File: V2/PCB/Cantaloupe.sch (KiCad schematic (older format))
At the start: 121 parts, among them J1 USB_In, J2 OLED, J3 Link, J4 Debug, J5 Trackball, Q1 2N7002, Q2 AO3401A, SW1 MX, SW10 MX, SW11 MX, SW12 MX, SW13 MX, SW14 MX, SW15 MX, SW16 MX, SW17 MX, SW18 MX, SW19 MX, SW2 MX, SW20 MX, SW21 MX, SW22 MX, SW23 MX, SW24 MX, SW25 MX, SW26 MX, SW27 MX, SW28 MX, SW29 MX, SW3 MX, SW30 MX, SW31 Encoder, SW32 MX, SW4 MX, SW5 MX, SW6 MX, SW7 MX, SW8 MX, SW9 MX, U1 STM32F4x1CxUx, U2 SRV0504, U3 SRV0504, U4 XC6206P332MR, U5 LMV321, Y1 8MHz

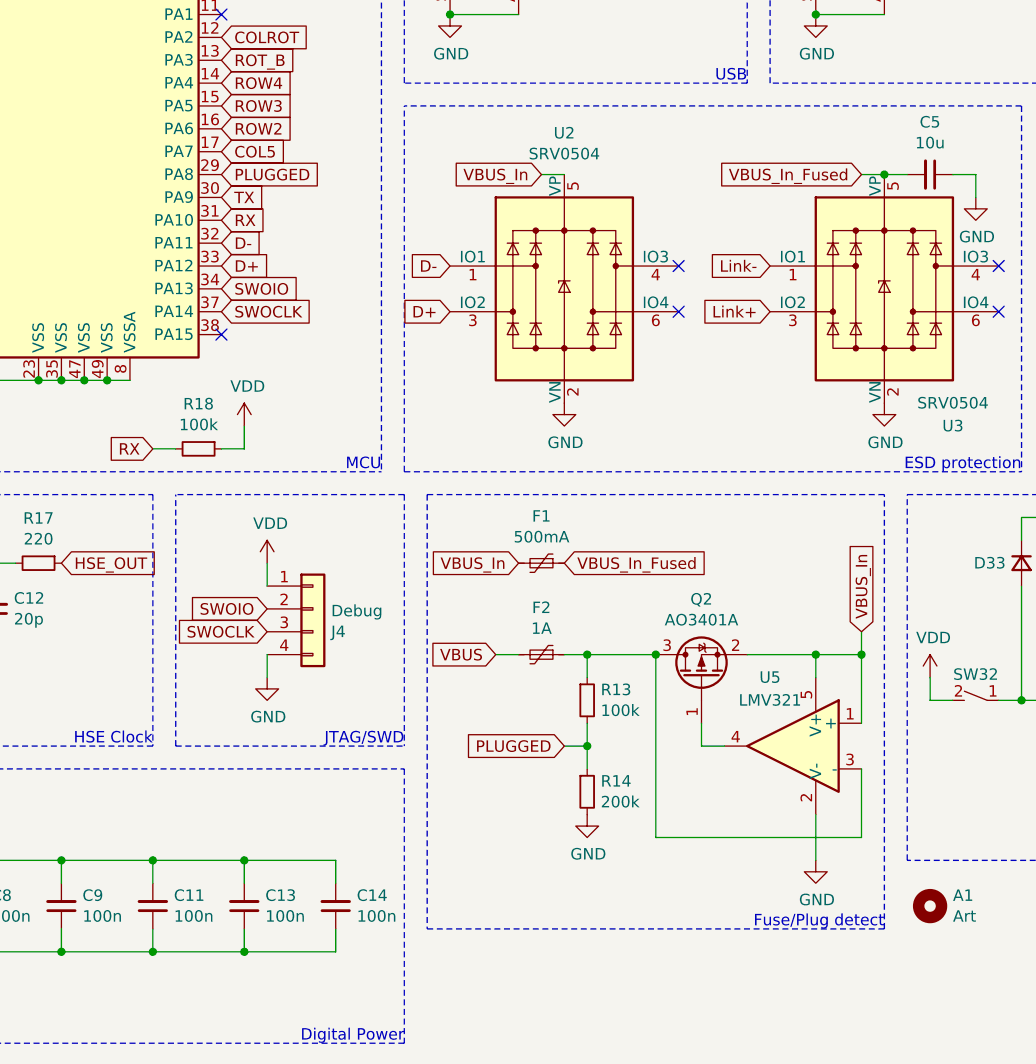
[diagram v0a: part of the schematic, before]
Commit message: Clean up of design. Added gerbers and files for FR4 plates.
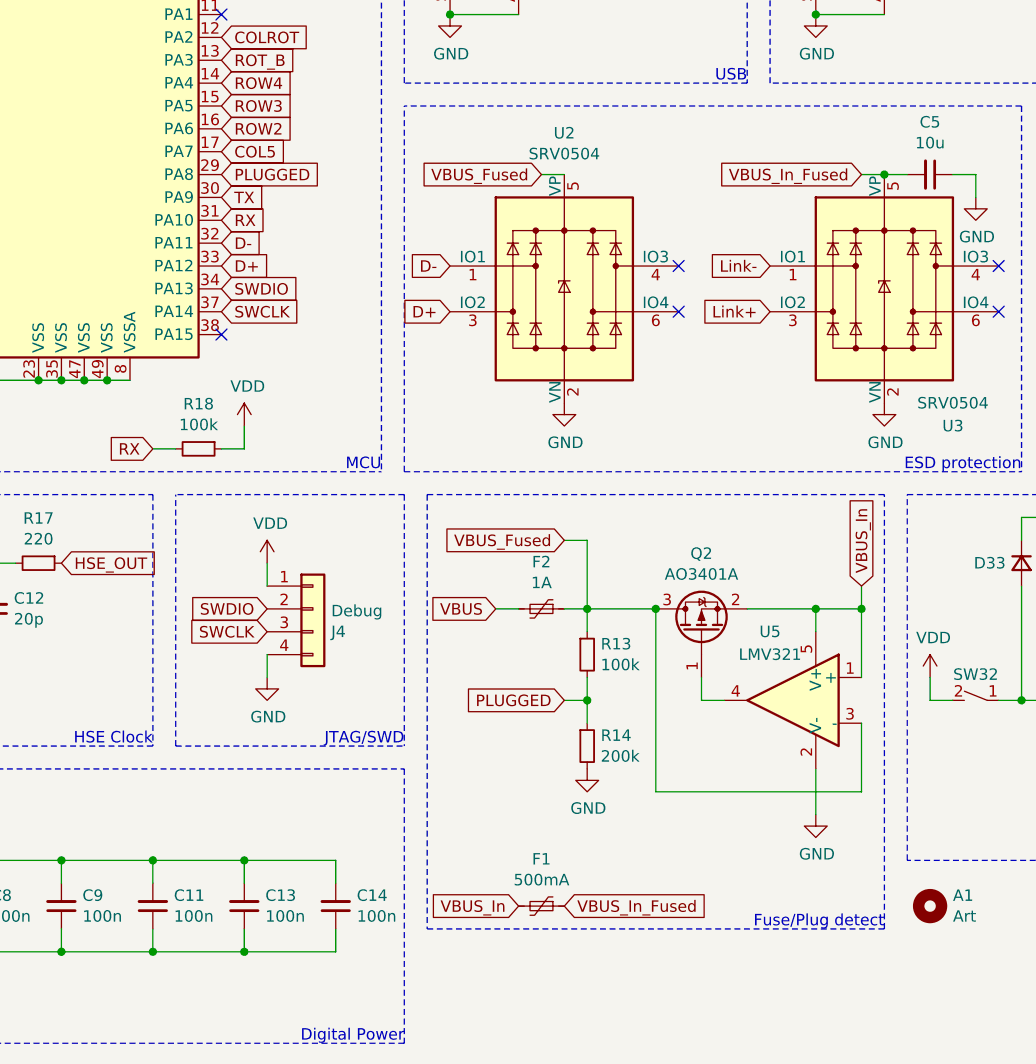
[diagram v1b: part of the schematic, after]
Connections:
- net VBUS_In: no longer U2.5 (VP)
- net VBUS_Fused: now reaches F2.1, Q2.3 (D), R13.1, U5.3 (-)
- net VBUS_Fused: now also U2.5 (VP)
- net SWOCLK renamed SWCLK
- net SWOIO renamed SWDIO
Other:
- moved on the sheet: F1, F2, Q2, R13, R14, U5
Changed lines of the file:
@@
 Wire Notes Line
 	2100 5800 6400 5800
-Text GLabel 6900 4900 0    50   Input ~ 0
+Text GLabel 6900 6400 0    50   Input ~ 0
 VBUS_In
 $Comp
 L Device:Polyfuse_Small F1
 U 1 1 6233E288
-P 7000 4900
-F 0 "F1" V 6795 4900 50  0000 C CNN
-F 1 "500mA" V 6886 4900 50  0000 C CNN
-F 2 "Fuse:Fuse_1206_3216Metric" H 7050 4700 50  0001 L CNN
-F 3 "~" H 7000 4900 50  0001 C CNN
-	1    7000 4900
+P 7000 6400
+F 0 "F1" V 6795 6400 50  0000 C CNN
+F 1 "500mA" V 6886 6400 50  0000 C CNN
+F 2 "Fuse:Fuse_1206_3216Metric" H 7050 6200 50  0001 L CNN
+F 3 "~" H 7000 6400 50  0001 C CNN
+	1    7000 6400
 	0    1    1    0
 $EndComp
-Text GLabel 7100 4900 2    50   Input ~ 0
+Text GLabel 7100 6400 2    50   Input ~ 0
 VBUS_In_Fused
 Text GLabel 9200 800  2    50   Input ~ 0
@@
 	4400 1000 4800 1000
 Text GLabel 5600 3700 2    50   Input ~ 0
-SWOIO
+SWDIO
 $Comp
 L MCU_ST_STM32F4:STM32F411CCUx U1
@@
 	10100 5200 10000 5200
 Text GLabel 5600 3800 2    50   Input ~ 0
-SWOCLK
+SWCLK
 NoConn ~ 5600 3900
 NoConn ~ 4300 2800
-Text GLabel 5800 5100 0    50   Input ~ 0
-SWOIO
-Text GLabel 5800 5200 0    50   Input ~ 0
-SWOCLK
 Wire Notes Line
 	6400 4600 5400 4600
@@
 NoConn ~ 9000 3600
 Text GLabel 7000 3200 0    50   Input ~ 0
-VBUS_In
+VBUS_Fused
 Connection ~ 8500 3200
 Wire Wire Line
@@
 Wire Notes Line
 	8500 6500 8500 4600
-Text GLabel 8400 5200 1    50   Input ~ 0
+Text GLabel 8400 5000 1    50   Input ~ 0
 VBUS_In
 Wire Wire Line
-	7700 5700 7700 5600
+	7700 5500 7700 5400
 $Comp
 L Transistor_FET:AO3401A Q2
 U 1 1 62437866
-P 7700 5400
-F 0 "Q2" V 8042 5400 50  0000 C CNN
-F 1 "AO3401A" V 7951 5400 50  0000 C CNN
-F 2 "Package_TO_SOT_SMD:SOT-23" H 7900 5325 50  0001 L CIN
-F 3 "http://www.aosmd.com/pdfs/datasheet/AO3401A.pdf" H 7700 5400 50  0001 L CNN
-	1    7700 5400
+P 7700 5200
+F 0 "Q2" V 8042 5200 50  0000 C CNN
+F 1 "AO3401A" V 7951 5200 50  0000 C CNN
+F 2 "Package_TO_SOT_SMD:SOT-23" H 7900 5125 50  0001 L CIN
+F 3 "http://www.aosmd.com/pdfs/datasheet/AO3401A.pdf" H 7700 5200 50  0001 L CNN
+	1    7700 5200
 	0    -1   -1   0
 $EndComp
 Wire Wire Line
-	7800 5700 7700 5700
-Wire Wire Line
-	7500 6100 8400 6100
+	7800 5500 7700 5500
+Wire Wire Line
+	7500 5900 8400 5900
 $Comp
 L power:GND #PWR0123
 U 1 1 631C4FB0
-P 8200 6200
-F 0 "#PWR0123" H 8200 5950 50  0001 C CNN
-F 1 "GND" H 8205 6027 50  0000 C CNN
-F 2 "" H 8200 6200 50  0001 C CNN
-F 3 "" H 8200 6200 50  0001 C CNN
-	1    8200 6200
-	1    0    0    -1
-$EndComp
-Wire Wire Line
-	8400 5200 8400 5300
-Connection ~ 8400 5300
-Wire Wire Line
-	8400 5800 8400 6100
-Wire Wire Line
-	8400 5600 8400 5300
-Wire Wire Line
-	7900 5300 8200 5300
-Connection ~ 8200 5300
-Wire Wire Line
-	8200 5300 8400 5300
-Wire Wire Line
-	8200 5400 8200 5300
-Wire Wire Line
-	8200 6000 8200 6200
-Wire Wire Line
-	7500 5300 7500 6100
+P 8200 6000
+F 0 "#PWR0123" H 8200 5750 50  0001 C CNN
+F 1 "GND" H 8205 5827 50  0000 C CNN
+F 2 "" H 8200 6000 50  0001 C CNN
+F 3 "" H 8200 6000 50  0001 C CNN
+	1    8200 6000
+	1    0    0    -1
+$EndComp
+Wire Wire Line
+	8400 5000 8400 5100
+Connection ~ 8400 5100
+Wire Wire Line
+	8400 5600 8400 5900
+Wire Wire Line
+	8400 5400 8400 5100
+Wire Wire Line
+	7900 5100 8200 5100
+Connection ~ 8200 5100
+Wire Wire Line
+	8200 5100 8400 5100
+Wire Wire Line
+	8200 5200 8200 5100
+Wire Wire Line
+	8200 5800 8200 6000
+Wire Wire Line
+	7500 5100 7500 5900
 $Comp
 L Amplifier_Operational:LMV321 U5
 U 1 1 62452FE5
-P 8100 5700
-F 0 "U5" H 8200 6000 50  0000 C CNN
-F 1 "LMV321" H 8200 5900 50  0000 C CNN
-F 2 "Package_TO_SOT_SMD:SOT-23-5" H 8100 5700 50  0001 L CNN
-F 3 "http://www.ti.com/lit/ds/symlink/lmv324.pdf" H 8100 5700 50  0001 C CNN
-	1    8100 5700
+P 8100 5500
+F 0 "U5" H 8200 5800 50  0000 C CNN
+F 1 "LMV321" H 8200 5700 50  0000 C CNN
+F 2 "Package_TO_SOT_SMD:SOT-23-5" H 8100 5500 50  0001 L CNN
+F 3 "http://www.ti.com/lit/ds/symlink/lmv324.pdf" H 8100 5500 50  0001 C CNN
+	1    8100 5500
 	-1   0    0    -1
 $EndComp
@@
 L Device:Polyfuse_Small F2
 U 1 1 6240F7C8
-P 7000 5300
-F 0 "F2" V 6795 5300 50  0000 C CNN
-F 1 "1A" V 6886 5300 50  0000 C CNN
-F 2 "Fuse:Fuse_1206_3216Metric" H 7050 5100 50  0001 L CNN
-F 3 "~" H 7000 5300 50  0001 C CNN
-	1    7000 5300
+P 7000 5100
+F 0 "F2" V 6795 5100 50  0000 C CNN
+F 1 "1A" V 6886 5100 50  0000 C CNN
+F 2 "Fuse:Fuse_1206_3216Metric" H 7050 4900 50  0001 L CNN
+F 3 "~" H 7000 5100 50  0001 C CNN
+	1    7000 5100
 	0    1    1    0
 $EndComp
 Wire Wire Line
-	6900 5300 6800 5300
-Text GLabel 6800 5300 0    50   Input ~ 0
+	6900 5100 6800 5100
+Text GLabel 6800 5100 0    50   Input ~ 0
 VBUS
-Connection ~ 7500 5300
-Wire Wire Line
-	7200 5300 7500 5300
-Wire Wire Line
-	7200 5300 7100 5300
-Connection ~ 7200 5300
-Wire Wire Line
-	7200 5400 7200 5300
+Connection ~ 7500 5100
+Wire Wire Line
+	7200 5100 7500 5100
+Wire Wire Line
+	7200 5100 7100 5100
+Connection ~ 7200 5100
+Wire Wire Line
+	7200 5200 7200 5100
 $Comp
 L power:GND #PWR0138
 U 1 1 62427BC2
-P 7200 6000
-F 0 "#PWR0138" H 7200 5750 50  0001 C CNN
-F 1 "GND" H 7205 5827 50  0000 C CNN
-F 2 "" H 7200 6000 50  0001 C CNN
-F 3 "" H 7200 6000 50  0001 C CNN
-	1    7200 6000
+P 7200 5800
+F 0 "#PWR0138" H 7200 5550 50  0001 C CNN
+F 1 "GND" H 7205 5627 50  0000 C CNN
+F 2 "" H 7200 5800 50  0001 C CNN
+F 3 "" H 7200 5800 50  0001 C CNN
+	1    7200 5800
 	1    0    0    -1
 $EndComp
@@
 L Device:R_Small R14
 U 1 1 6250C728
-P 7200 5900
-F 0 "R14" H 7259 5946 50  0000 L CNN
-F 1 "200k" H 7259 5855 50  0000 L CNN
-F 2 "Resistor_SMD:R_0603_1608Metric" H 7200 5900 50  0001 C CNN
-F 3 "~" H 7200 5900 50  0001 C CNN
-	1    7200 5900
-	1    0    0    -1
-$EndComp
-Wire Wire Line
-	7200 5800 7200 5700
-Wire Wire Line
-	7200 5700 7200 5600
-Connection ~ 7200 5700
-Wire Wire Line
-	7100 5700 7200 5700
-Text GLabel 7100 5700 0    50   Input ~ 0
+P 7200 5700
+F 0 "R14" H 7259 5746 50  0000 L CNN
+F 1 "200k" H 7259 5655 50  0000 L CNN
+F 2 "Resistor_SMD:R_0603_1608Metric" H 7200 5700 50  0001 C CNN
+F 3 "~" H 7200 5700 50  0001 C CNN
+	1    7200 5700
+	1    0    0    -1
+$EndComp
+Wire Wire Line
+	7200 5600 7200 5500
+Wire Wire Line
+	7200 5500 7200 5400
+Connection ~ 7200 5500
+Wire Wire Line
+	7100 5500 7200 5500
+Text GLabel 7100 5500 0    50   Input ~ 0
 PLUGGED
 $Comp
 L Device:R_Small R13
 U 1 1 624179D2
-P 7200 5500
-F 0 "R13" H 7259 5546 50  0000 L CNN
-F 1 "100k" H 7259 5455 50  0000 L CNN
-F 2 "Resistor_SMD:R_0603_1608Metric" H 7200 5500 50  0001 C CNN
-F 3 "~" H 7200 5500 50  0001 C CNN
-	1    7200 5500
+P 7200 5300
+F 0 "R13" H 7259 5346 50  0000 L CNN
+F 1 "100k" H 7259 5255 50  0000 L CNN
+F 2 "Resistor_SMD:R_0603_1608Metric" H 7200 5300 50  0001 C CNN
+F 3 "~" H 7200 5300 50  0001 C CNN
+	1    7200 5300
 	1    0    0    -1
 $EndComp
 Text GLabel 5600 3200 2    50   Input ~ 0
 PLUGGED
+Text GLabel 7100 4800 0    50   Input ~ 0
+VBUS_Fused
+Wire Wire Line
+	7200 5100 7200 4800
+Wire Wire Line
+	7200 4800 7100 4800
+Text GLabel 5800 5100 0    50   Input ~ 0
+SWDIO
+Text GLabel 5800 5200 0    50   Input ~ 0
+SWCLK
 $EndSCHEMATC
